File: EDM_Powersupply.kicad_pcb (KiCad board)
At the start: 2 copper layers, 116.5 x 85 mm, 41 parts, among them IC1 ACSL-7210-06RE, J1 Conn_01x13_Pin, J2 Screw_Terminal_01x02, J3 Screw_Terminal_01x02, J4 Screw_Terminal_01x02, J5 Screw_Terminal_01x02, J6 Conn_01x07_Pin, J7 Conn_01x03_Pin, Q1 IPW65R037C6, U1 MGJ2D241505SC, U2 L7805, U3 STGAP2SM, U4 RASPBERRY_PI_PICO, U5 TLV3501AID, U6 MGJ2D241505SC

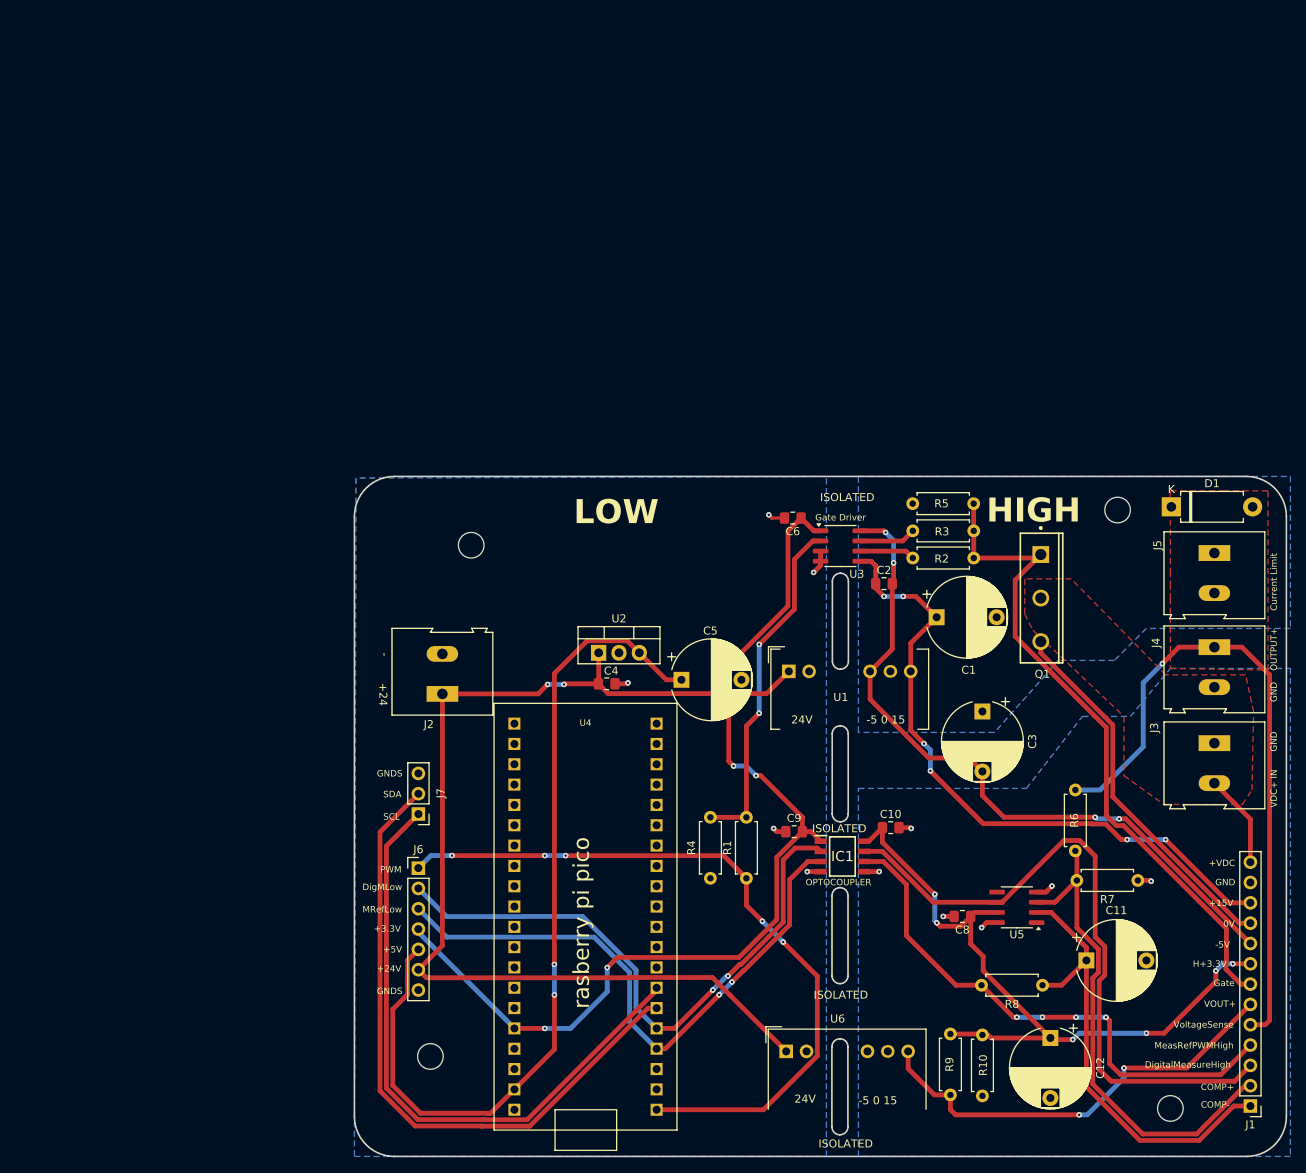
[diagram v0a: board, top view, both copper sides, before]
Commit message: stash
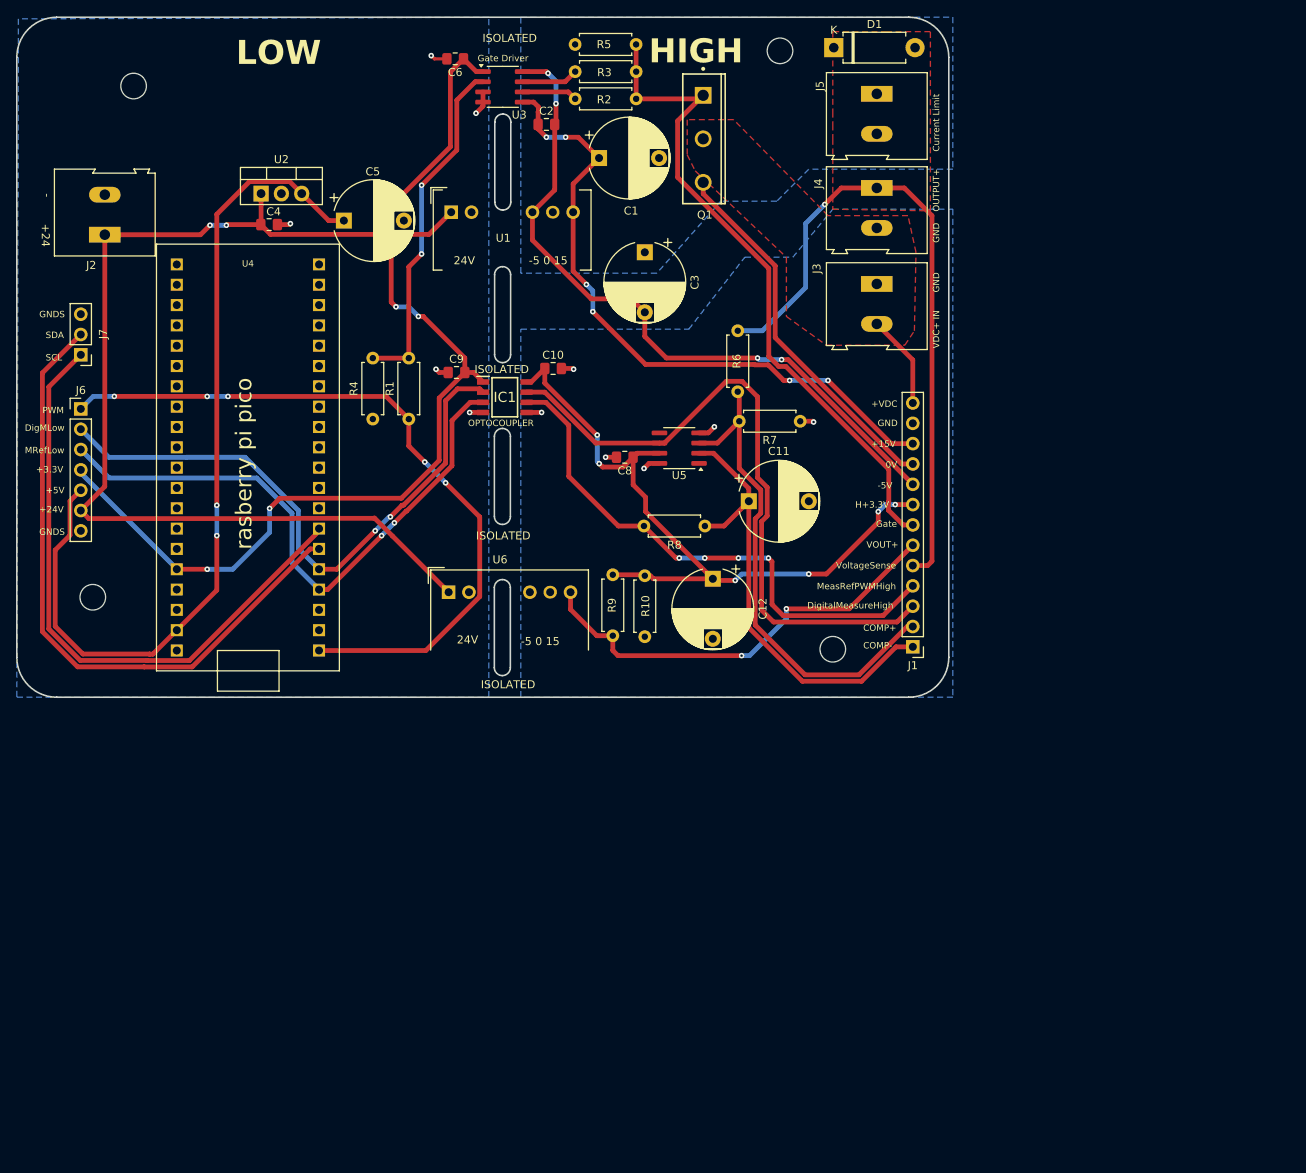
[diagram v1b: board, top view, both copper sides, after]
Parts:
- moved C11 71.2 mm to (111.3, 79.1)
- moved C6 71.2 mm to (74.6, 23.8)
- moved C8 71.2 mm to (95.8, 73.6)
- moved H1 71.2 mm to (29.3, 91.1)
- moved H2 71.2 mm to (121.8, 97.6)
- moved H3 71.2 mm to (115.2, 22.8)
- moved IC1 71.2 mm to (80.8, 66.1)
- moved J2 71.2 mm to (30.8, 45.8)
- moved J3 71.2 mm to (127.3, 51.9)
- moved J4 71.2 mm to (127.3, 39.9)
- moved J5 71.2 mm to (127.3, 28.2)
- moved J7 71.2 mm to (27.8, 60.8)
- moved Q1 71.2 mm to (105.6, 33.8)
- moved R1 71.2 mm to (68.8, 68.8)
- moved R10 71.2 mm to (98.3, 88.4)
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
